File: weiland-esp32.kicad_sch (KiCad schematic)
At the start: 38 parts, among them J1 S02B-PASK-2, J6 S02B-PASK-2, J7 S02B-PASK-2, P1 S04B-PASK-2_LF__SN_, P2 S04B-PASK-2_LF__SN_, U1 ESP32-WROOM-32E(8MB), U2 AMS1117-3.3_C347222, U3 MAX98357AETE_T, U5 ULN2003F12FN-7, U6 DZ127S-22-06-55

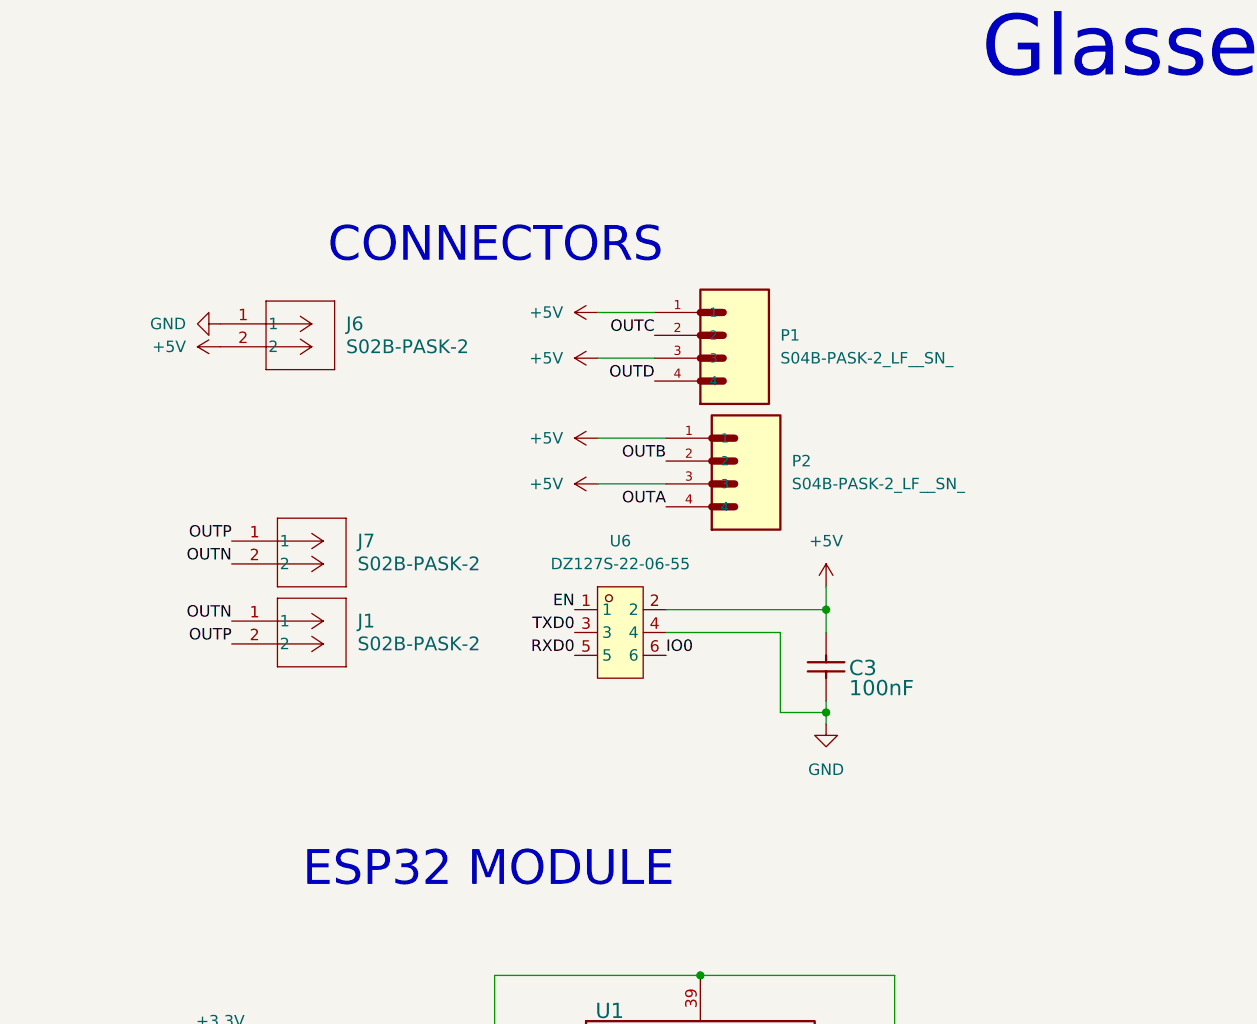
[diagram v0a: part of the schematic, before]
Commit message: latest
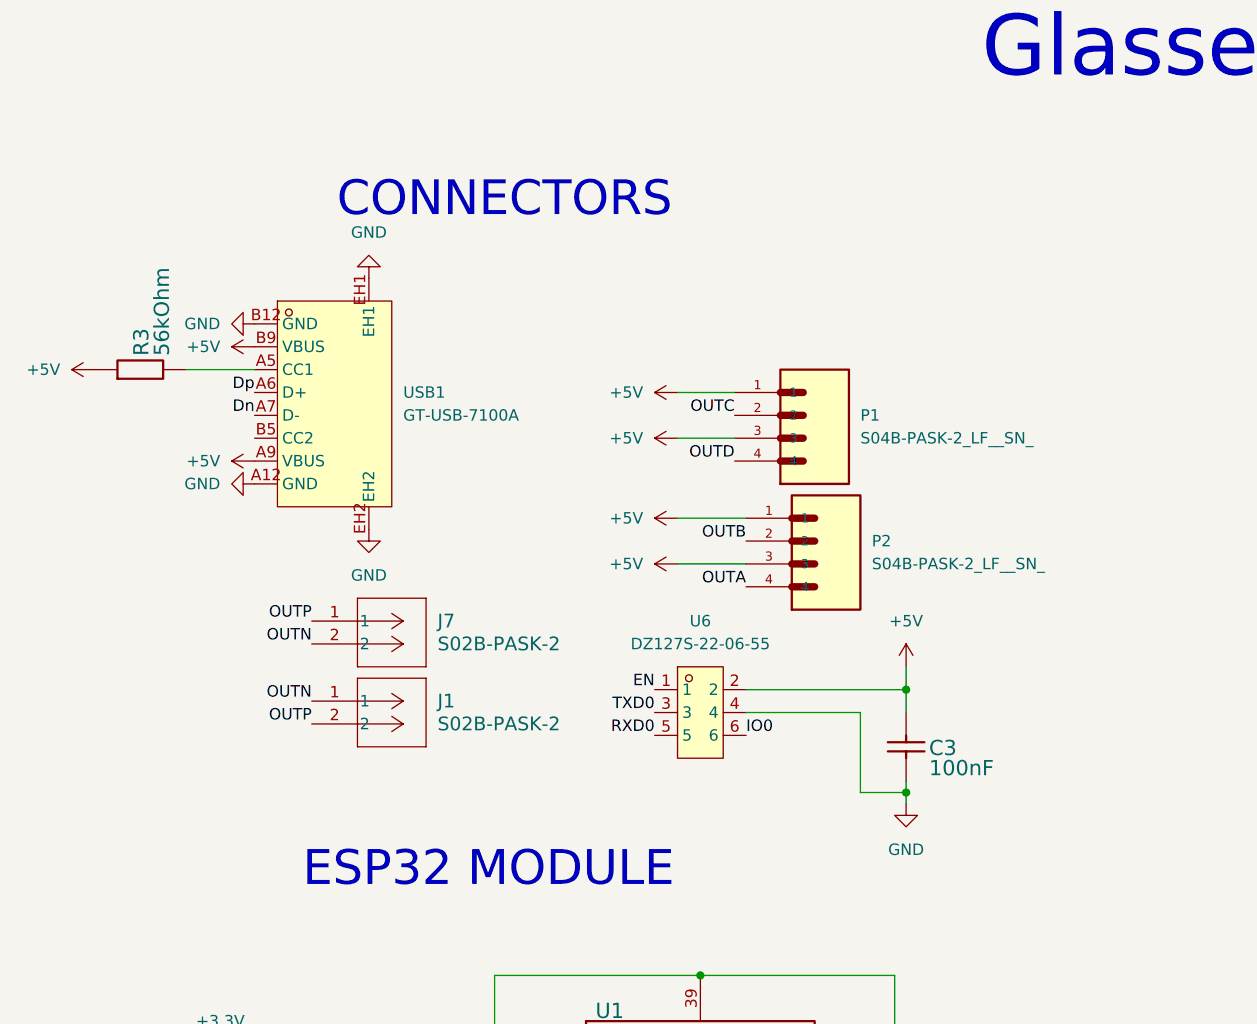
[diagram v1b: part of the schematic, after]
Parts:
- removed J6: S02B-PASK-2, footprints:CONN2_S02B-PASK-2_JST, symbol jst2pin:S02B-PASK-2
- added R3: 56kOhm, Resistor_SMD:R_0402_1005Metric, symbol 0402WGF5101TCE
- added USB1: GT-USB-7100A, easyeda2kicad:USB-C-SMD_GT-USB-7100A, symbol easyeda2kicad:GT-USB-7100A
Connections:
- net +5V: now also R3.2, USB1.A9 (VBUS), USB1.B9 (VBUS)
- net GND: now also USB1.A12 (GND), USB1.B12 (GND), USB1.EH1, USB1.EH2
- new net: R3.1, USB1.A5 (CC1)
- new net Dn: USB1.A7 (D-)
- new net Dp: USB1.A6 (D+)
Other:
- moved on the sheet: C3, J1, J7, P1, P2, U6

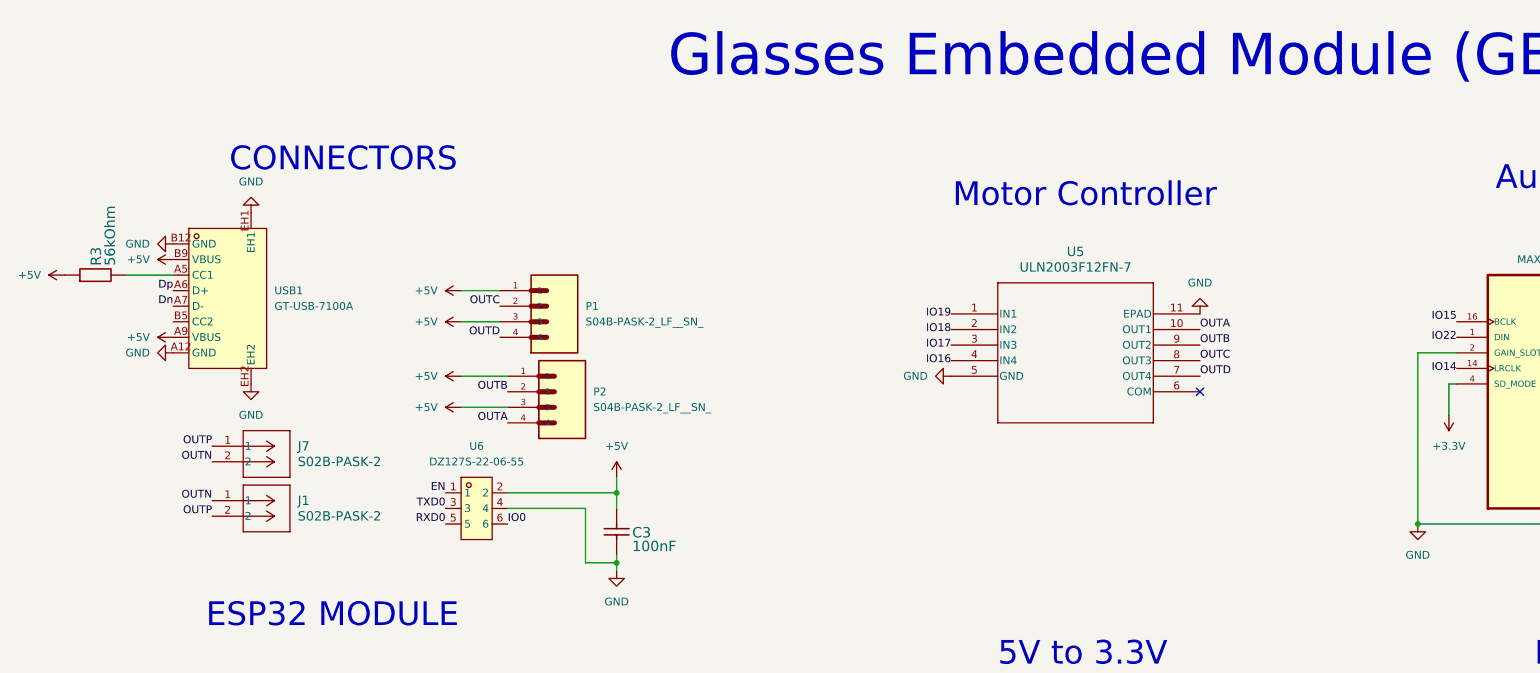
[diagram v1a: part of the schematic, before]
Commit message: test
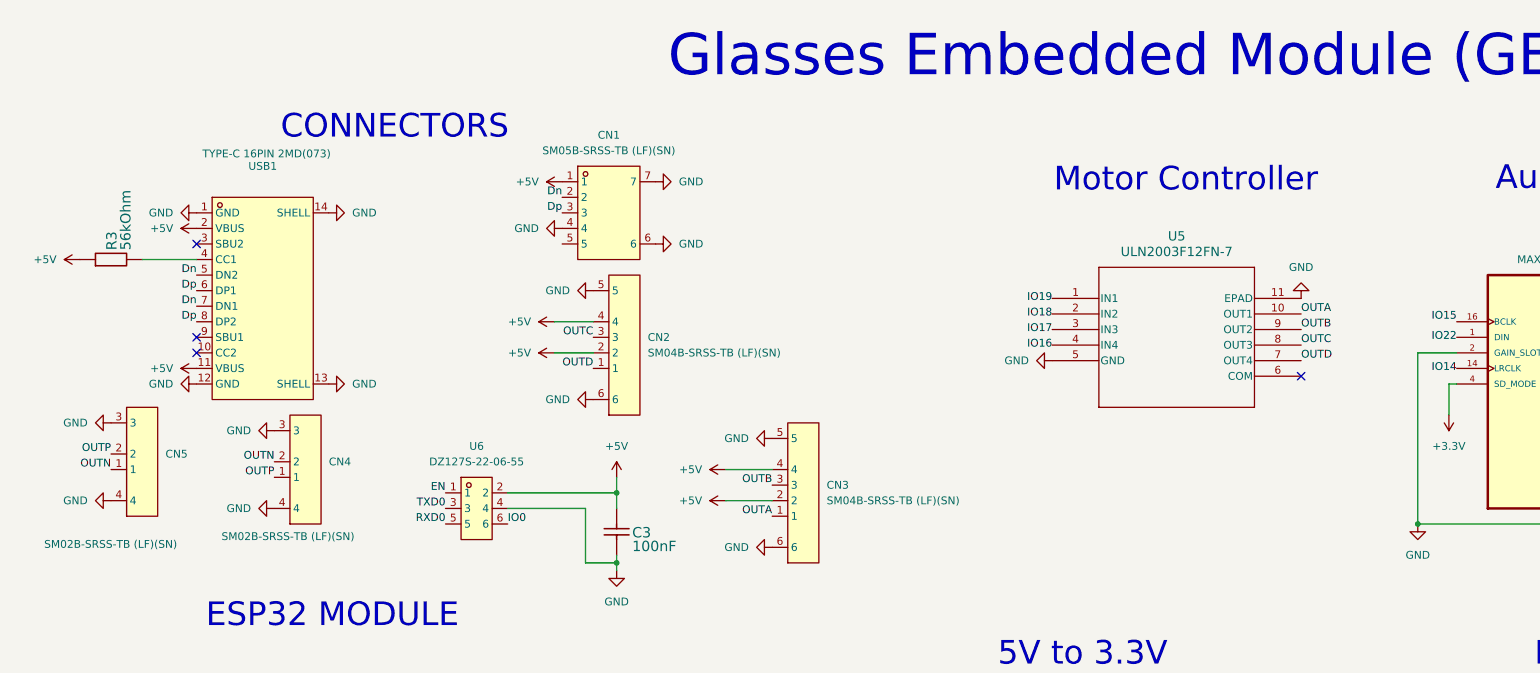
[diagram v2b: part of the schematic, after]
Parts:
- removed J1, J7: S02B-PASK-2, footprints:CONN2_S02B-PASK-2_JST, symbol jst2pin:S02B-PASK-2
- removed P1, P2: S04B-PASK-2_LF__SN_, S04B-PASK-2_LF__SN_:JST_S04B-PASK-2, symbol S04B-PASK-2:S04B-PASK-2_LF__SN_
- removed USB1: GT-USB-7100A, easyeda2kicad:USB-C-SMD_GT-USB-7100A, symbol easyeda2kicad:GT-USB-7100A
- added CN1: SM05B-SRSS-TB (LF)(SN), easyeda2kicad:CONN-SMD_SM05B-SRSS-TB-LF-SN, symbol easyeda2kicad:SM05B-SRSS-TB(LF)(SN)
- added CN2, CN3: SM04B-SRSS-TB (LF)(SN), easyeda2kicad:CONN-SMD_4P-P1.00_SM04B-SRSS-TB-LF-SN, symbol easyeda2kicad:SM04B-SRSS-TB(LF)(SN)
- added CN4, CN5: SM02B-SRSS-TB (LF)(SN), easyeda2kicad:CONN-SMD_2P-P1.00_SM02B-SRSS-TB-LF-SN, symbol easyeda2kicad:SM02B-SRSS-TB(LF)(SN)
- added USB1: TYPE-C 16PIN 2MD(073), easyeda2kicad:USB-C-SMD_TYPE-C-6PIN-2MD-073, symbol easyeda2kicad:TYPE-C16PIN2MD(073)
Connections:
- net +5V: now also CN1.1, CN2.2, CN2.4, CN3.2, CN3.4, USB1.11 (VBUS), USB1.2 (VBUS)
- net Dn: now also CN1.2, USB1.5 (DN2), USB1.7 (DN1)
- net Dp: now also CN1.3, USB1.6 (DP1), USB1.8 (DP2)
- net GND: now also CN1.4, CN1.6, CN1.7, CN2.5, CN2.6, CN3.5, CN3.6, CN4.3, CN4.4, CN5.3, CN5.4, USB1.1 (GND), USB1.12 (GND), USB1.13 (SHELL), USB1.14 (SHELL)
- net OUTA: now also CN3.1
- net OUTB: now also CN3.3
- net OUTC: now also CN2.3
- net OUTD: now also CN2.1
- net OUTN: now also CN4.2, CN5.1
- net OUTP: now also CN4.1, CN5.2
- net at R3.1: now also USB1.4 (CC1)
- no-connect marks 24 -> 27
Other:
- moved on the sheet: R3, U5
